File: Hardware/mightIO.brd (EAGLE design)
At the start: 37.8 x 31.7 mm, 47 parts, among them IC1 TL064D, IC2 TL064D, IC3 LM4041A12DBZ, U1 MAX11612

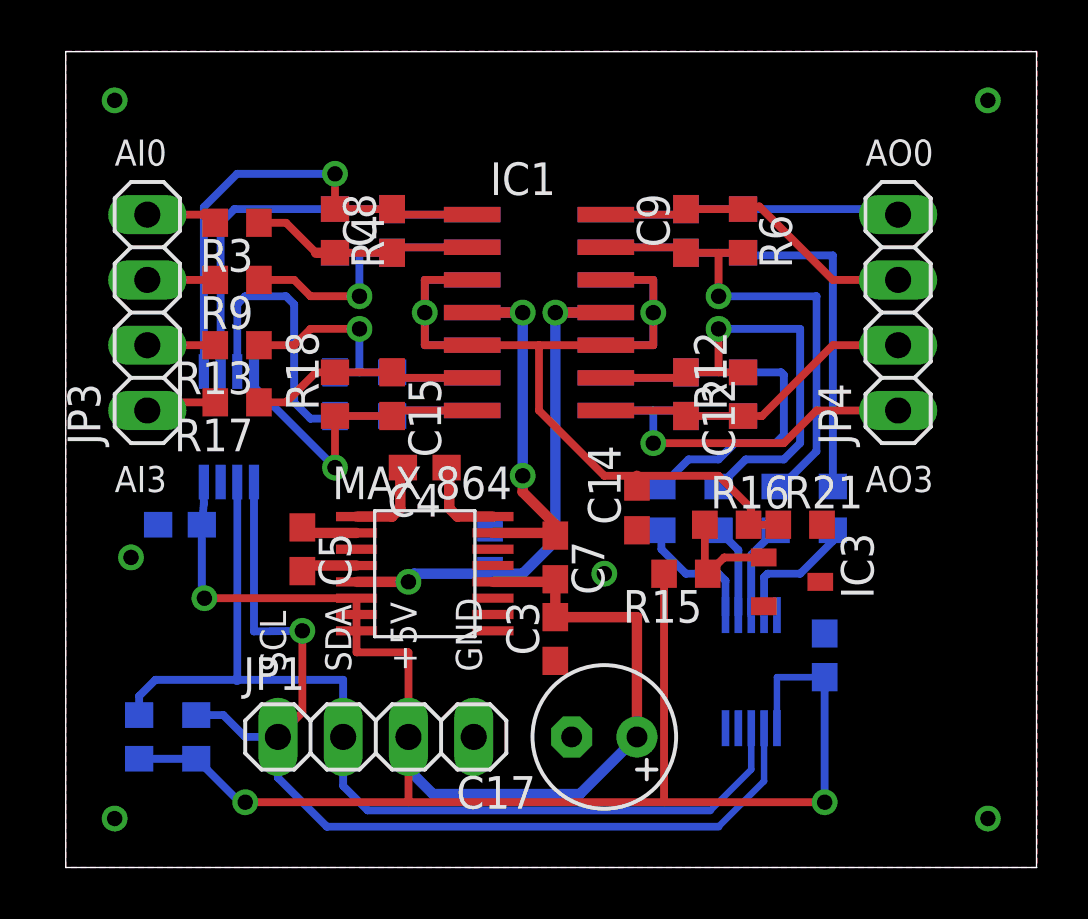
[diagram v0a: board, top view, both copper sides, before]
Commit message: Gerber files done
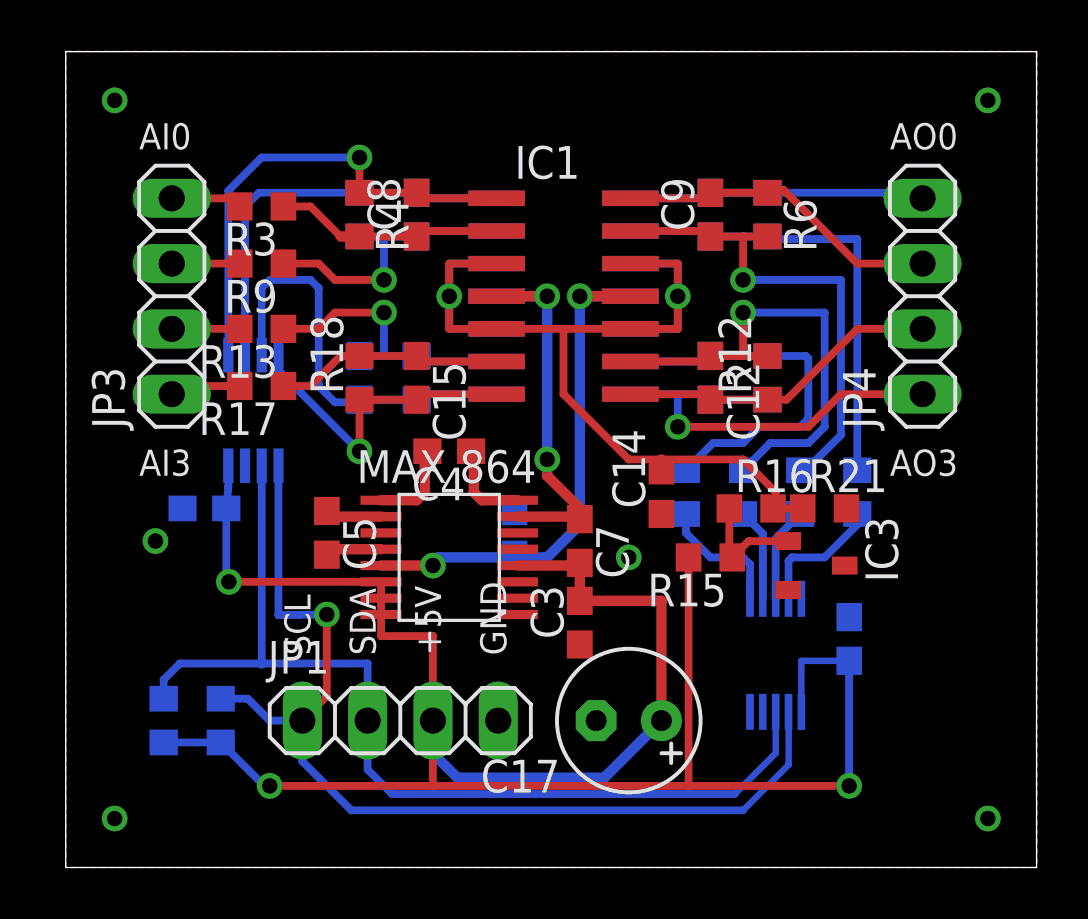
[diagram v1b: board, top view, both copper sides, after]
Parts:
- moved C10 1.14 mm to (25.1, 19.1)
- moved C12 1.14 mm to (25.1, 19.1)
- moved C13 1.14 mm to (11.4, 19.1)
- moved C15 1.14 mm to (13.7, 19.1)
- moved IC1 1.14 mm to (19.4, 22.2)
- moved IC2 1.14 mm to (19.4, 22.2)
- moved JP3 1.14 mm to (4.13, 22.2)
- moved JP4 1.14 mm to (33.3, 22.2)
- moved R12 1.14 mm to (27.3, 19.1)
- moved R14 1.14 mm to (13.7, 19.1)
- moved R18 1.14 mm to (11.4, 19.1)
- moved R8 1.14 mm to (27.3, 19.1)
- moved U1 1.14 mm to (7.30, 17.8)
- moved C17 1.14 mm to (21.9, 5.71)
- moved C2 1.14 mm to (30.5, 8.89)
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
